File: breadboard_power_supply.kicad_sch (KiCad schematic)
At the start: 15 parts, among them J1 Barrel_Jack_Switch, J4 Screw_Terminal_01x02, J5 Conn_01x03_Male, J6 Conn_01x03_Male, J7 Screw_Terminal_01x02, U1 LM7805_TO220, U2 LM317_TO-220

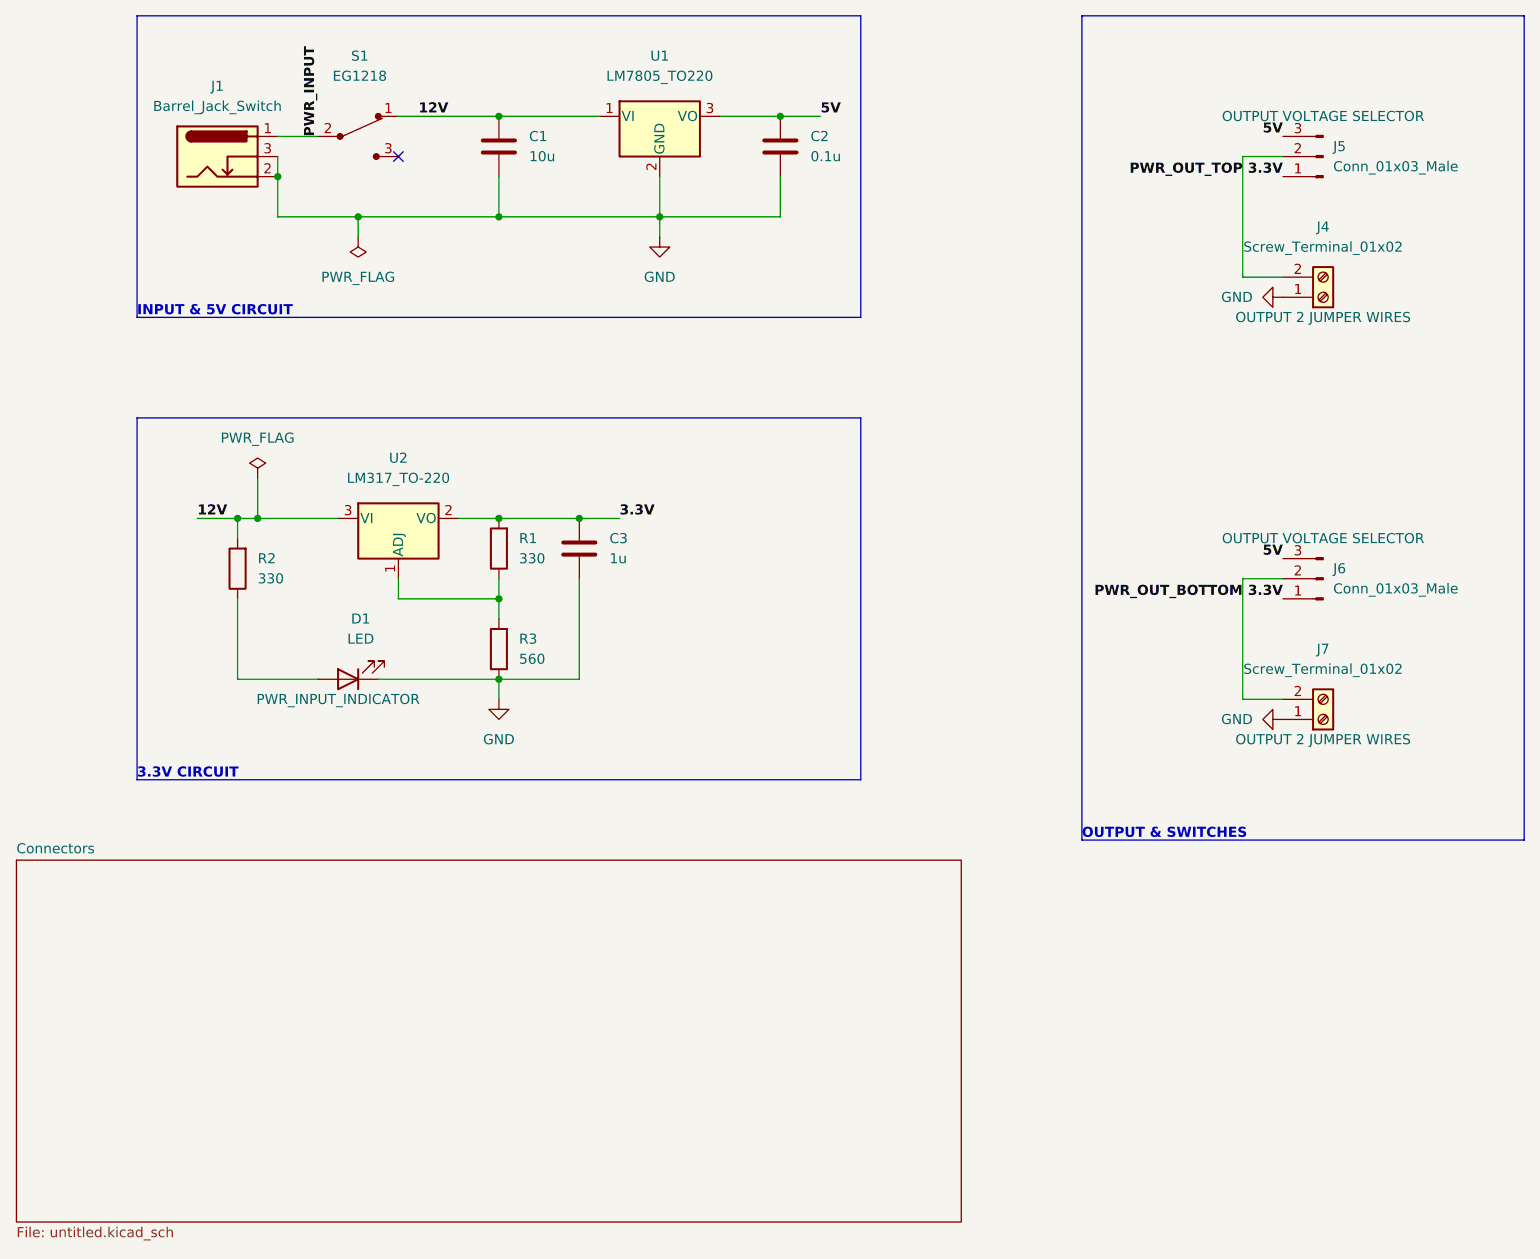
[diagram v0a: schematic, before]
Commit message: Revert "Project Target Description"
This reverts commit 992a993e3ba41f038e621602d57108eb9190e08b.
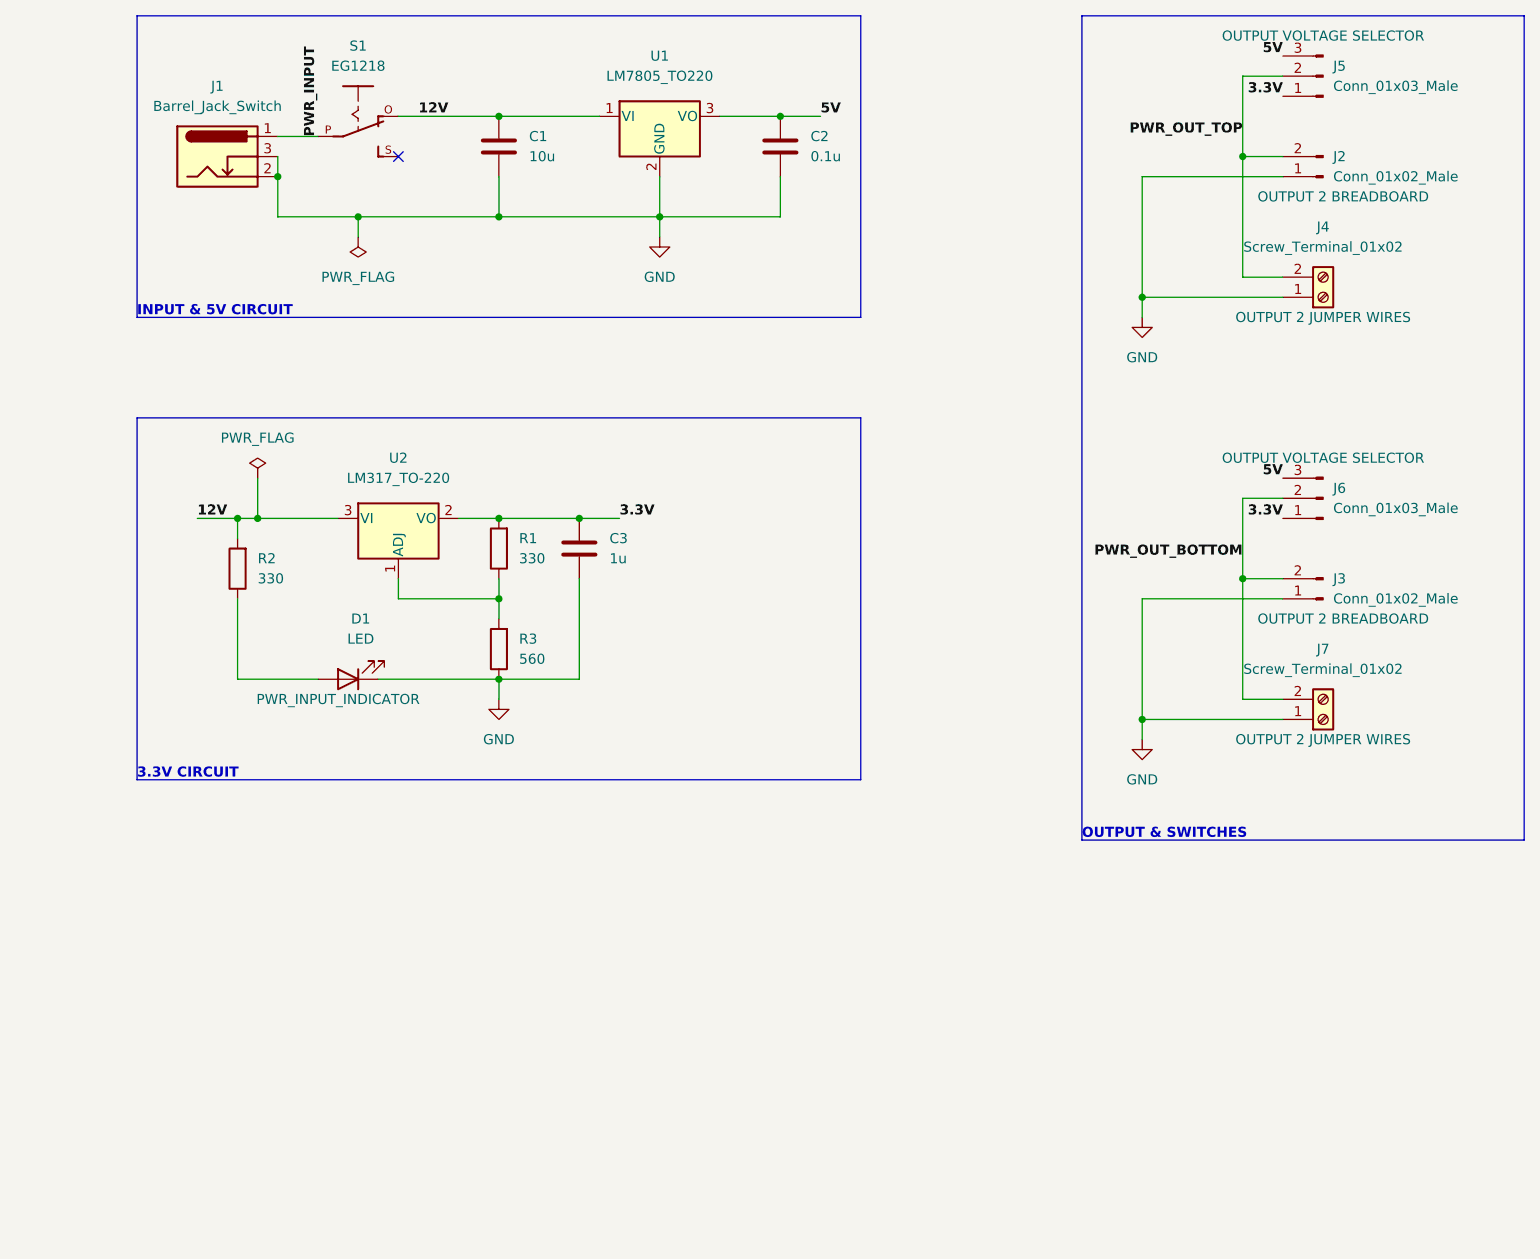
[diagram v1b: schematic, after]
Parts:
- removed S1: EG1218, digkey_slide_switch:Switch_Slide_11.6x4mm_EG1218, symbol digkey_slide_switch:EG1218
- added J2, J3: Conn_01x02_Male, Connector_PinHeader_2.54mm:PinHeader_1x02_P2.54mm_Vertical, symbol Connector:Conn_01x02_Male
- added S1: EG1218, EG1218:EG1218, symbol Slide_Switch:EG1218
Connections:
- net 12V: now also S1.O
- net GND: now also J2.1 (Pin_1), J3.1 (Pin_1)
- net PWR_INPUT: now also S1.P
- net PWR_OUT_BOTTOM: now also J3.2 (Pin_2)
- net PWR_OUT_TOP: now also J2.2 (Pin_2)
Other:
- removed sheet Connectors
- moved on the sheet: J5, J6
